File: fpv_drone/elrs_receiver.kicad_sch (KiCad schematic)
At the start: 12 parts, among them U2 ATmega32U4-A, Y1 16MHz

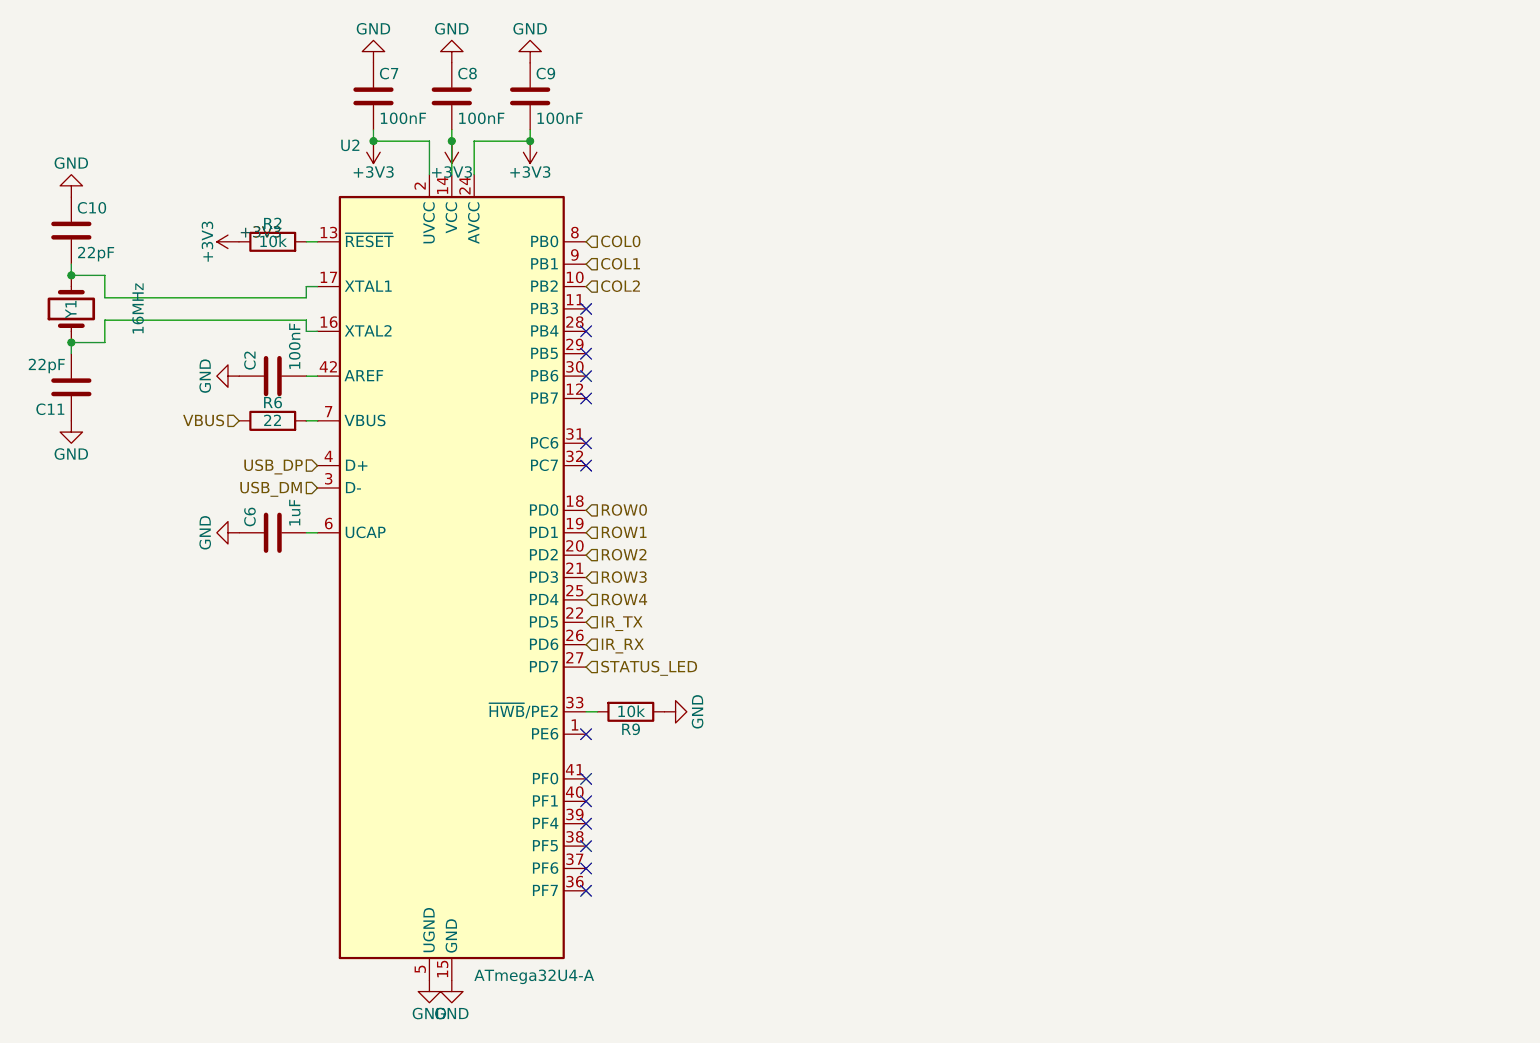
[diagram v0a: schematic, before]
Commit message: new boards
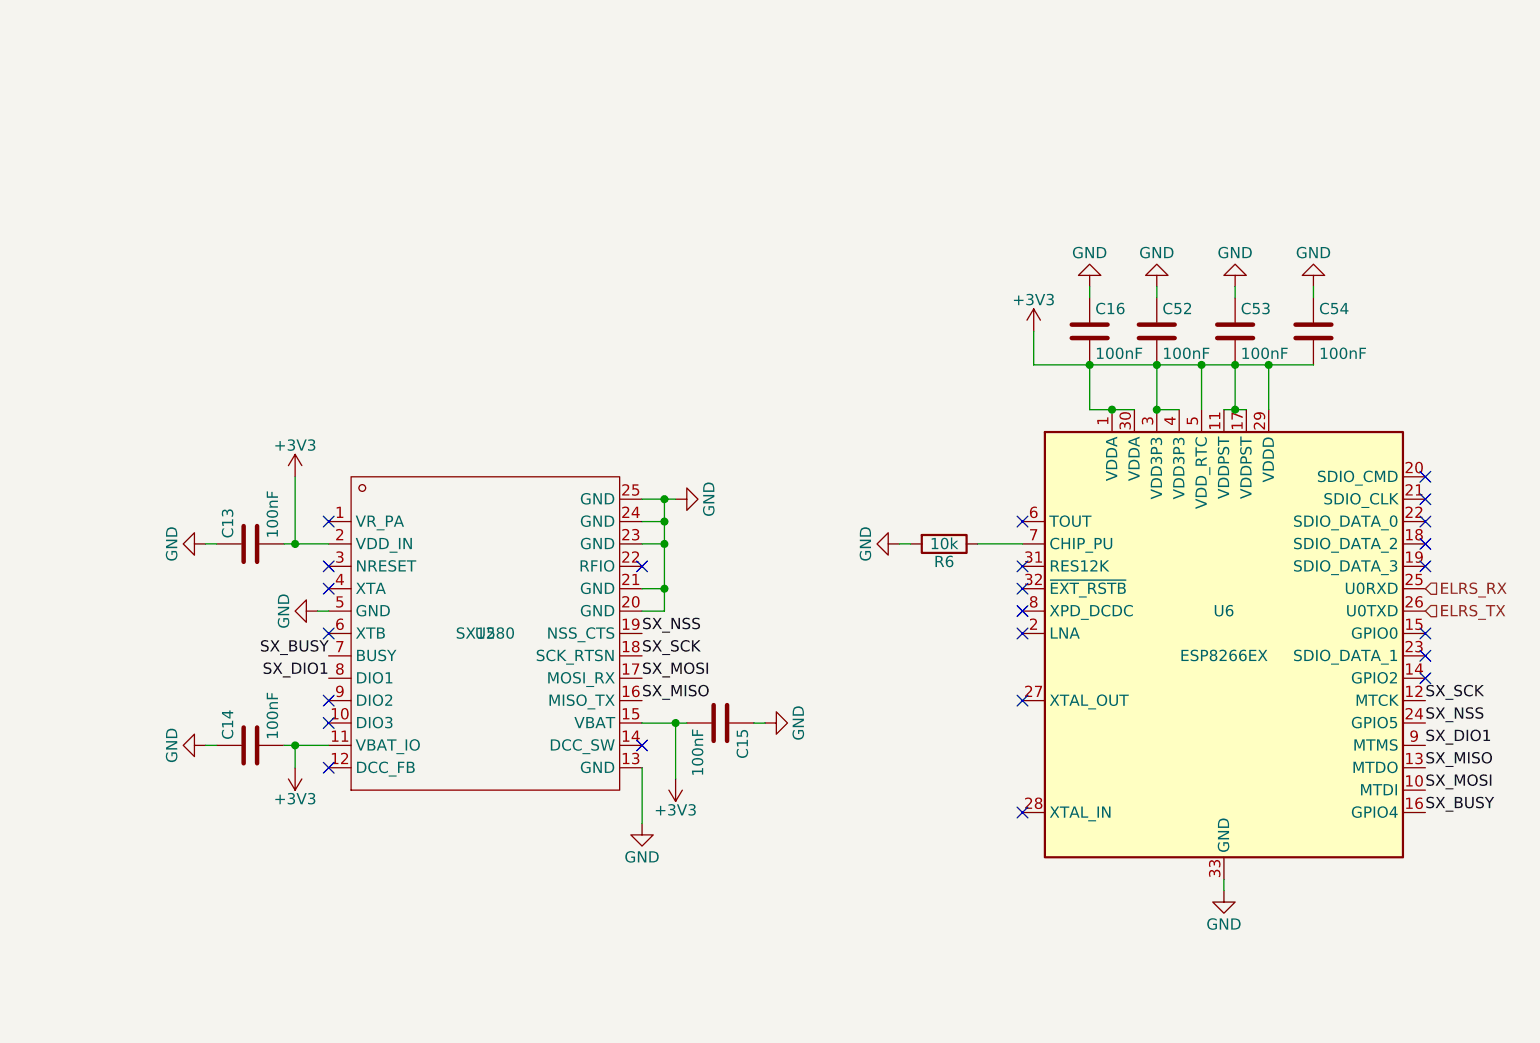
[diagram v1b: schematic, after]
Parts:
- removed C10, C11: 22pF, Capacitor_SMD:C_0402_1005Metric, symbol Device:C
- removed C2, C7, C8, C9: 100nF, Capacitor_SMD:C_0402_1005Metric, symbol Device:C
- removed C6: 1uF, Capacitor_SMD:C_0402_1005Metric, symbol Device:C
- removed R2, R9: 10k, Resistor_SMD:R_0402_1005Metric, symbol Device:R
- removed U2: ATmega32U4-A, Package_QFP:TQFP-44_10x10mm_P0.8mm, symbol MCU_Microchip_ATmega:ATmega32U4-A
- removed Y1: 16MHz, Crystal:Crystal_SMD_HC49-SD, symbol Device:Crystal
- added C13, C14, C15, C16, C52, C53, C54: 100nF, Capacitor_SMD:C_0402_1005Metric, symbol Device:C
- added U5: SX1280, SX1280IMLTRT:QFN-24_L4.0-W4.0-P0.50-BL-EP2.6, symbol SX1280IMLTRT:SX1280IMLTRT
- added U6: ESP8266EX, Package_DFN_QFN:QFN-32-1EP_5x5mm_P0.5mm_EP3.45x3.45mm, symbol MCU_Espressif:ESP8266EX
- R6: value 22 -> 10k
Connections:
- net +3V3: now also C13.2, C14.2, C15.2, C16.2, C52.2, C53.2, C54.2, U5.11 (VBAT_IO), U5.15 (VBAT), U5.2 (VDD_IN), U6.1 (VDDA), U6.11 (VDDPST), U6.17 (VDDPST), U6.29 (VDDD), U6.3 (VDD3P3), U6.30 (VDDA), U6.4 (VDD3P3), U6.5 (VDD_RTC)
- net GND: now also R6.2, C13.1, C14.1, C15.1, C16.1, C52.1, C53.1, C54.1, U5.13 (GND), U5.20 (GND), U5.21 (GND), U5.23 (GND), U5.24 (GND), U5.25 (GND), U5.5 (GND), U6.33 (GND)
- net VBUS: no longer names the net of R6.1
- net VBUS: now also U6.7 (CHIP_PU)
- new net ELRS_RX: U6.25 (U0RXD)
- new net ELRS_TX: U6.26 (U0TXD)
- new net SX_BUSY: U5.7 (BUSY), U6.16 (GPIO4)
- new net SX_DIO1: U5.8 (DIO1), U6.9 (MTMS)
- new net SX_MISO: U5.16 (MISO_TX), U6.13 (MTDO)
- new net SX_MOSI: U5.17 (MOSI_RX), U6.10 (MTDI)
- new net SX_NSS: U5.19 (NSS_CTS), U6.24 (GPIO5)
- new net SX_SCK: U5.18 (SCK_RTSN), U6.12 (MTCK)
- no-connect marks 14 -> 24
